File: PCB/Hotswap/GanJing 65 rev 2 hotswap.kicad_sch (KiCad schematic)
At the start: 151 parts, among them SW1 EC11_rotary_encoder, U1 Elite-C

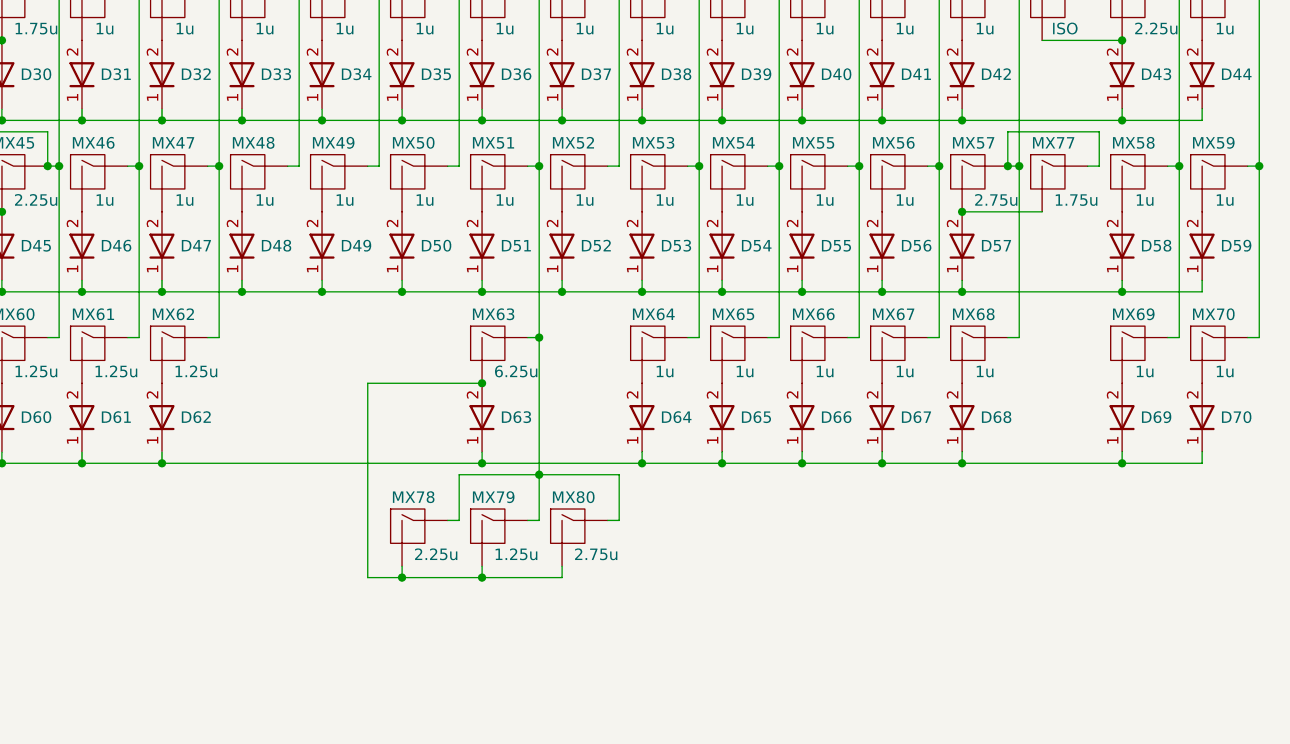
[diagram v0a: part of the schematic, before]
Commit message: Updating PCB and firmware
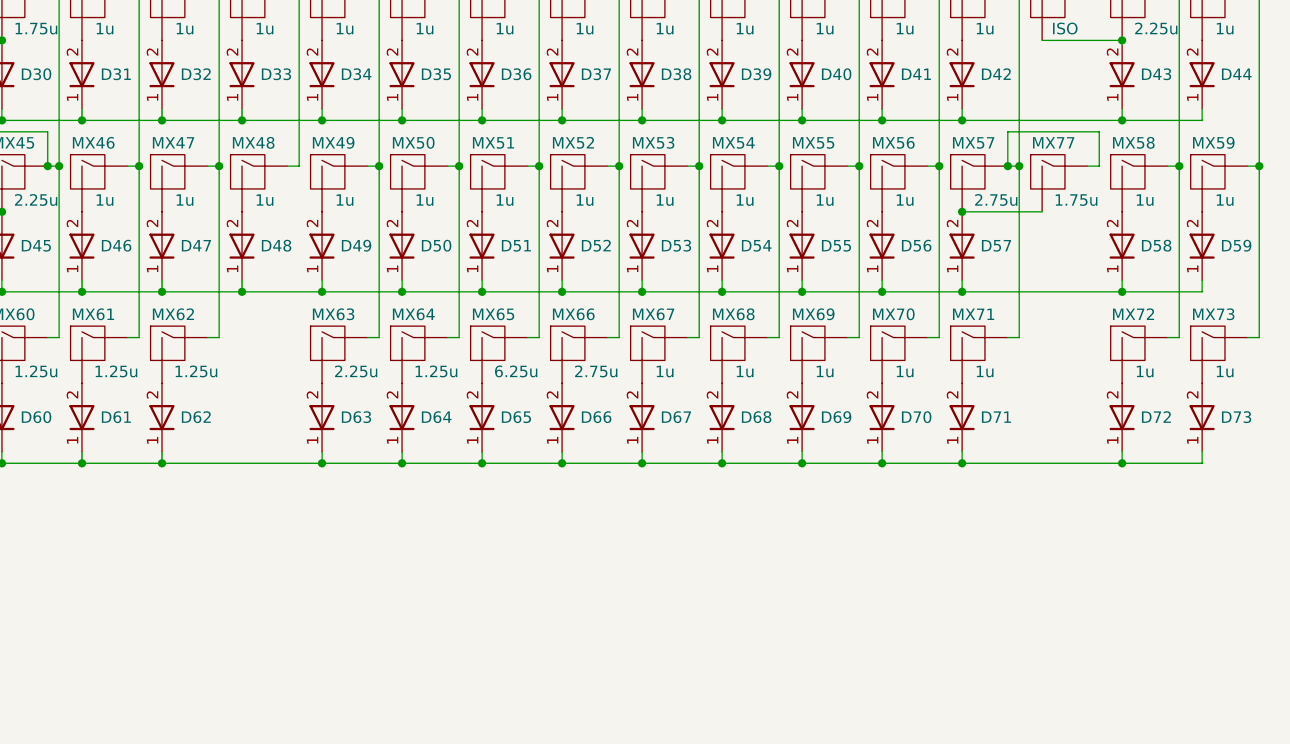
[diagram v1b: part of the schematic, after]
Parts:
- added D63, D64, D66: 1N4148TR_diode, GanJing_components:1N4148TR_diode, symbol GanJing_components:1N4148TR_diode
- renumbered D63 to D65, D64 to D67, D65 to D68, D66 to D69, D67 to D70, D68 to D71, D69 to D72, D70 to D73, MX78 to MX63, MX79 to MX64, MX63 to MX65, MX80 to MX66, MX64 to MX67, MX65 to MX68, MX66 to MX69, MX67 to MX70, MX68 to MX71, MX69 to MX72, MX70 to MX73
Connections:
- net col_5: now also MX63.1 (COL)
- net col_6: now also MX64.1 (COL)
- net col_7: no longer MX63.1 (COL), MX64.1 (COL), MX66.1 (COL)
- net col_8: now also MX66.1 (COL)
- net row_5: now also D63.1, D64.1, D66.1
- new net: D65.2, MX65.2 (ROW)
- new net: D64.2, MX64.2 (ROW)
- new net: D63.2, MX63.2 (ROW)
- new net: D66.2, MX66.2 (ROW)
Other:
- moved on the sheet: MX63, MX64, MX66
